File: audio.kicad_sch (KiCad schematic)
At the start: 5 parts, among them J6 AudioJack3

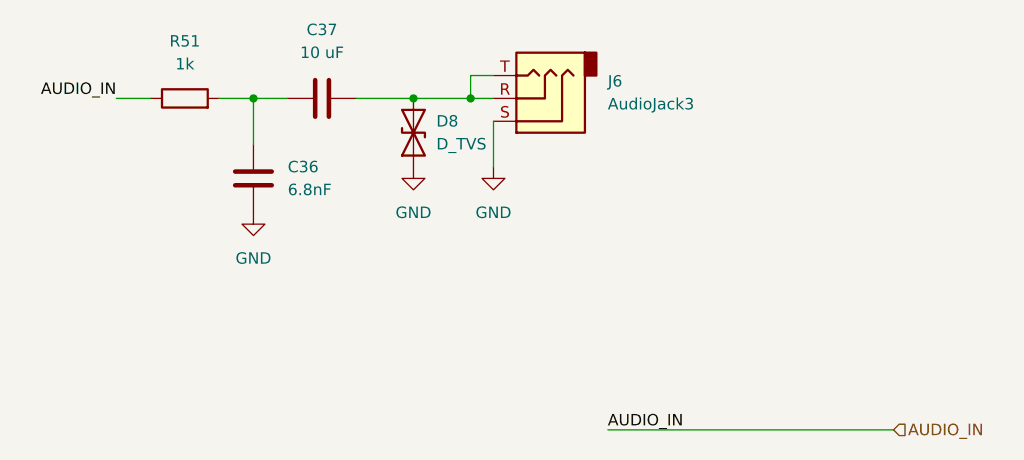
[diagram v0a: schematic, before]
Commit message: fixed several issues from review
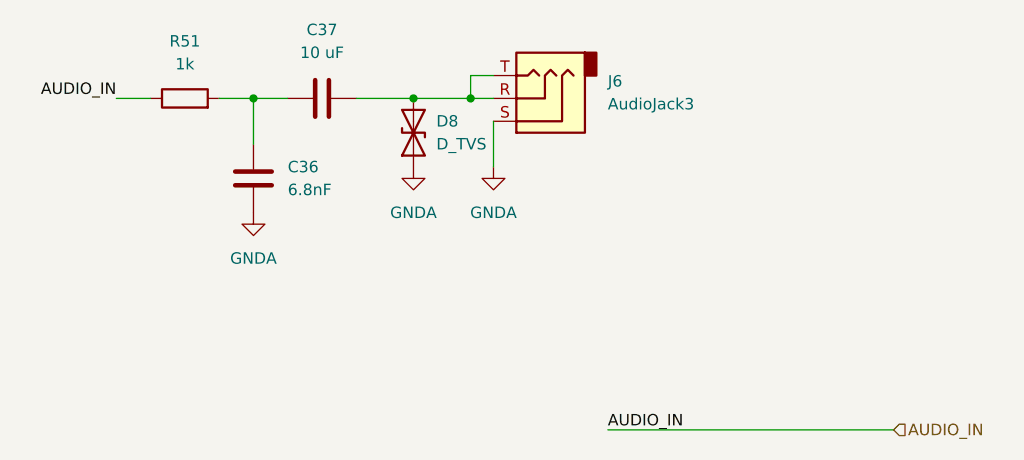
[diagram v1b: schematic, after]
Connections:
- net GND renamed GNDA
